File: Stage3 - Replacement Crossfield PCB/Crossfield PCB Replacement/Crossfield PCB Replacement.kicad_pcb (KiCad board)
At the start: 2 copper layers, 29 parts, among them P16-2 Power Amp Right, P21 4_Way_215079-4, P25-2 Power Amp Left, P6-P18 12_Way_8-215079-2, Q1 BC549, Q2 BC557, Q3 BC557, Q4 BC557

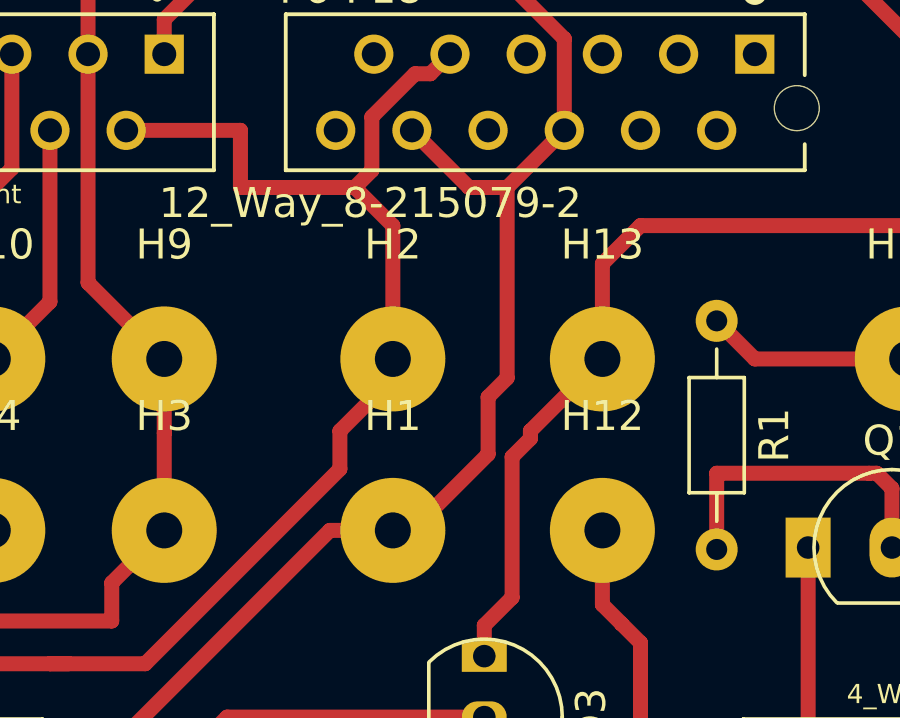
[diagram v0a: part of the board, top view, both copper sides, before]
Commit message: PCB tweaks
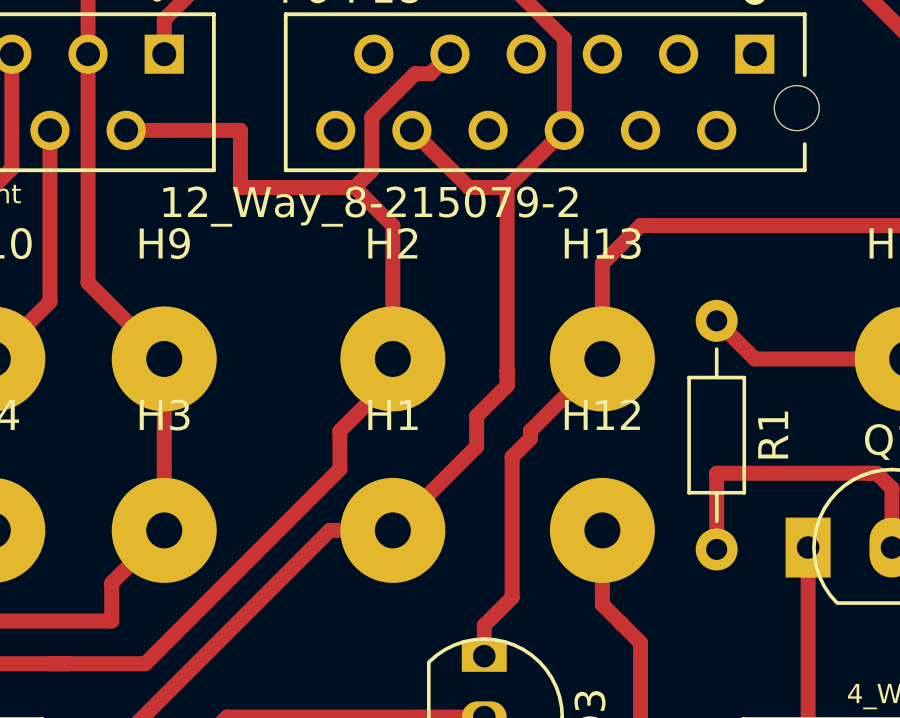
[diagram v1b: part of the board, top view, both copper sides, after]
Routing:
- net /+9V: track 56.4 -> 56.9 mm
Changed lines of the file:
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@@
     (thickness 1.6)
     (drawings 4)
-    (tracks 189)
+    (tracks 191)
     (zones 0)
     (modules 29)
@@
   (segment (start 146.685 85.09) (end 146.685 83.936) (width 0.5) (layer F.Cu) (net 1))
   (segment (start 157.991922 82.55) (end 149.225 82.55) (width 0.5) (layer F.Cu) (net 1))
-  (segment (start 154.94 100.965) (end 157.48 98.425) (width 0.5) (layer F.Cu) (net 1))
-  (segment (start 157.48 98.425) (end 157.48 96.52) (width 0.5) (layer F.Cu) (net 1))
-  (segment (start 157.48 96.52) (end 158.115 95.885) (width 0.5) (layer F.Cu) (net 1))
   (segment (start 158.115 89.535) (end 160.02 87.63) (width 0.5) (layer F.Cu) (net 1))
-  (segment (start 158.115 95.885) (end 158.115 89.535) (width 0.5) (layer F.Cu) (net 1))
   (segment (start 156.845 89.535) (end 158.115 89.535) (width 0.5) (layer F.Cu) (net 1))
   (segment (start 154.94 87.63) (end 156.845 89.535) (width 0.5) (layer F.Cu) (net 1))
+  (segment (start 158.115 95.631) (end 158.115 96.139) (width 0.5) (layer F.Cu) (net 1))
+  (segment (start 158.115 95.631) (end 158.115 89.535) (width 0.5) (layer F.Cu) (net 1))
+  (segment (start 158.115 95.885) (end 158.115 95.631) (width 0.5) (layer F.Cu) (net 1))
+  (segment (start 158.115 96.139) (end 157.099 97.155) (width 0.5) (layer F.Cu) (net 1))
+  (segment (start 157.099 98.171) (end 154.305 100.965) (width 0.5) (layer F.Cu) (net 1))
+  (segment (start 157.099 97.155) (end 157.099 98.171) (width 0.5) (layer F.Cu) (net 1))
   (segment (start 139.7 111.125) (end 139.7 105.41) (width 0.5) (layer F.Cu) (net 10))
   (segment (start 152.539939 97.650061) (end 152.539939 98.920061) (width 0.5) (layer F.Cu) (net 10))
